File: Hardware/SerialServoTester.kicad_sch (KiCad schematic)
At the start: 12 parts, among them J1 Conn_01x04_Pin, J2 Screw_Terminal_01x02, P1 USB_C_Plug_USB2.0, Q1 BSS84, U1 FT230XS, U2 LT1785AxN8

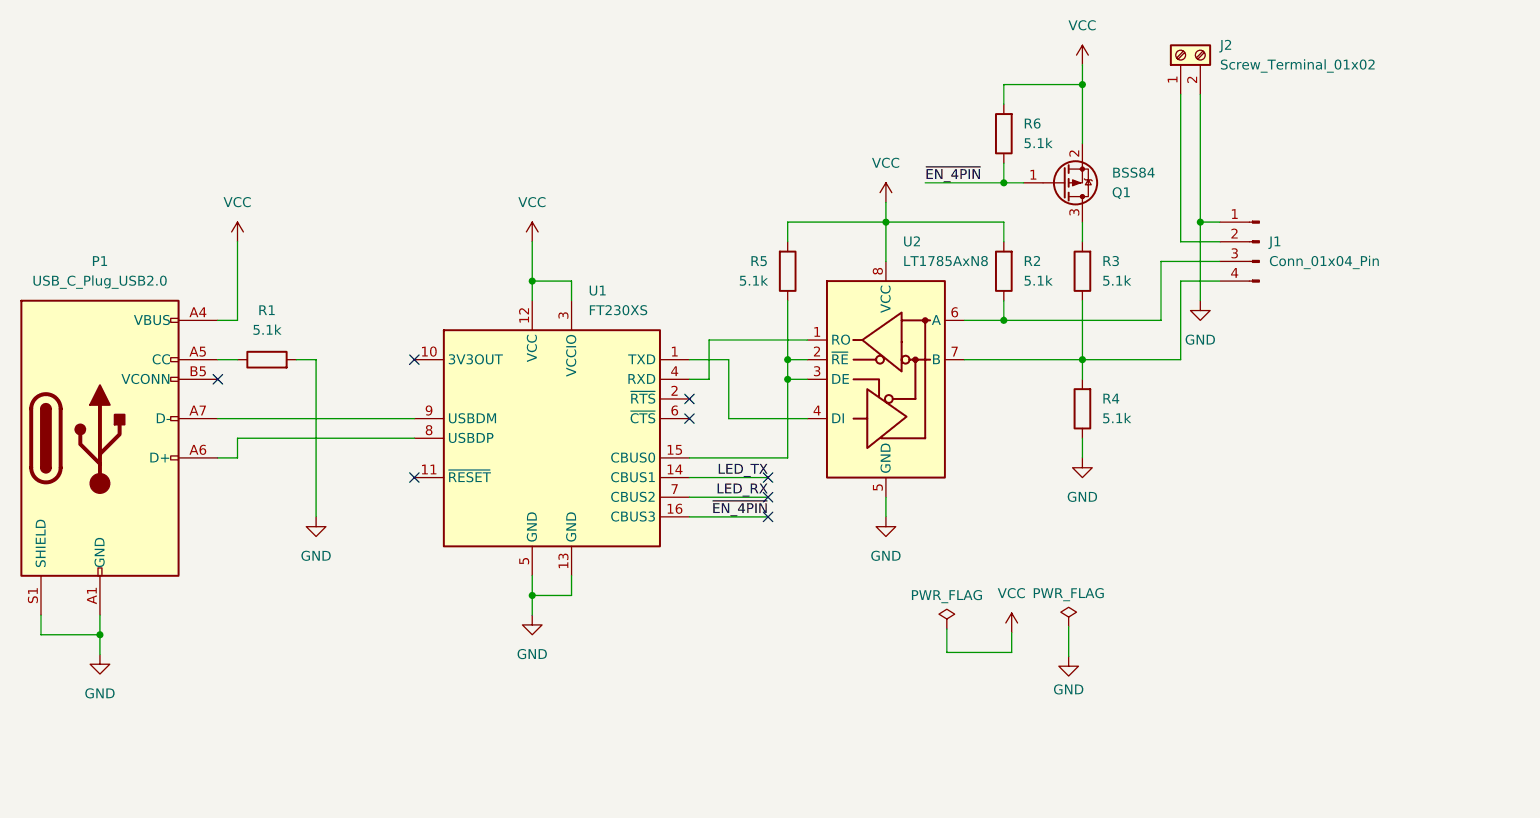
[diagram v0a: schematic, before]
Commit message: Update PCB design
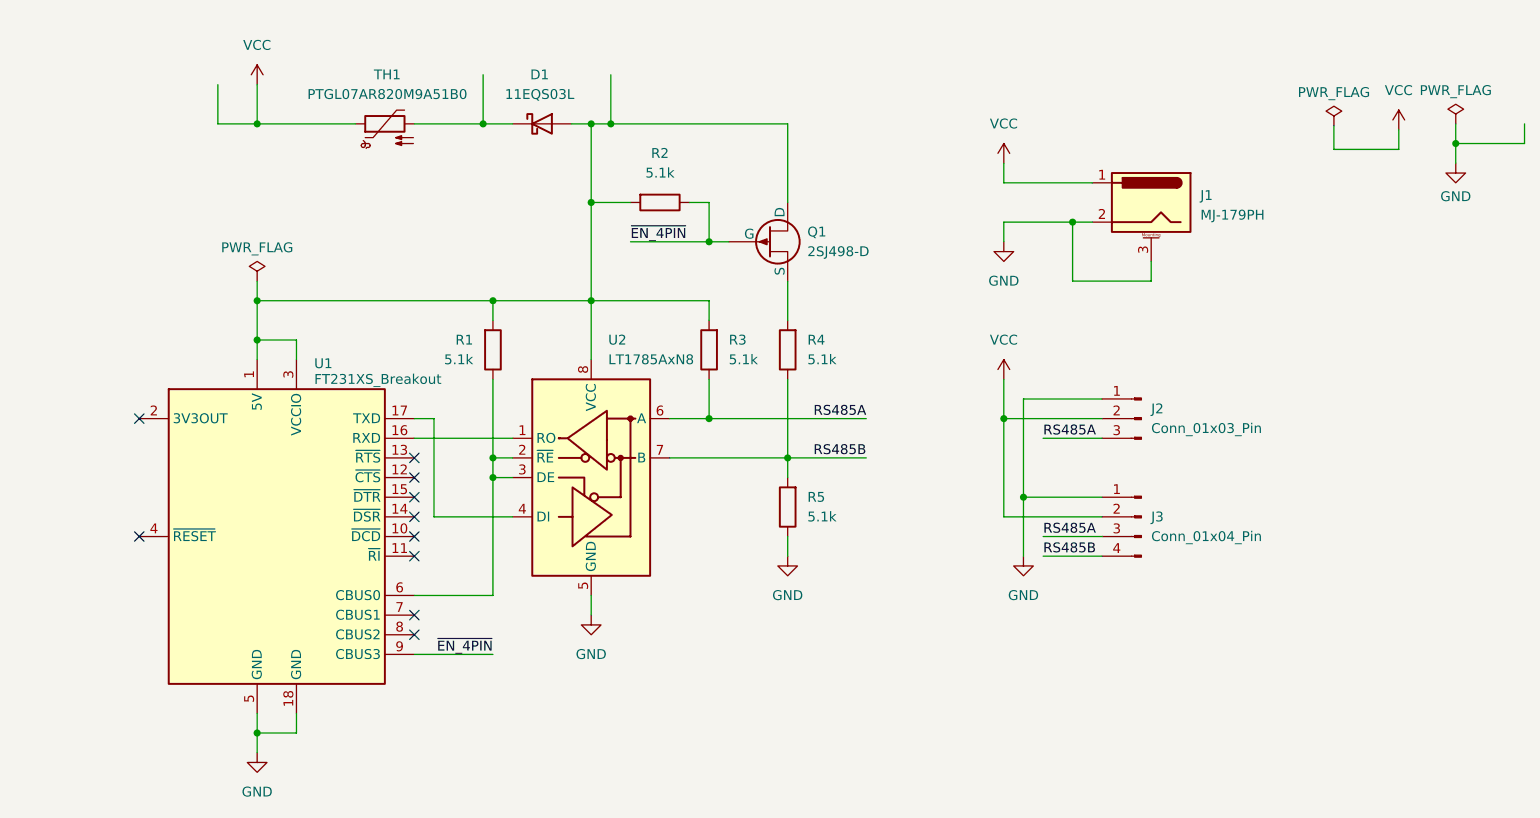
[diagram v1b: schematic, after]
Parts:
- removed J2: Screw_Terminal_01x02, TerminalBlock:TerminalBlock_bornier-2_P5.08mm, symbol Connector:Screw_Terminal_01x02
- removed P1: USB_C_Plug_USB2.0, Connector_USB:USB_C_Plug_JAE_DX07P024AJ1, symbol Connector:USB_C_Plug_USB2.0
- removed Q1: BSS84, Package_TO_SOT_SMD:SOT-23, symbol Transistor_FET:BSS84
- removed R1, R6: 5.1k, Resistor_SMD:R_0603_1608Metric_Pad0.98x0.95mm_HandSolder, symbol Device:R
- removed U1: FT230XS, Package_SO:SSOP-16_3.9x4.9mm_P0.635mm, symbol Interface_USB:FT230XS
- added D1: 11EQS03L, Diode_THT:D_T-1_P10.16mm_Horizontal, symbol Device:D_Schottky
- added J1: MJ-179PH, Connector_BarrelJack:BarrelJack_Horizontal, symbol Connector:Barrel_Jack_MountingPin
- added J2: Conn_01x03_Pin, Connector_PinHeader_2.54mm:PinHeader_1x03_P2.54mm_Horizontal, symbol Connector:Conn_01x03_Pin
- added Q1: 2SJ498-D, Package_TO_SOT_THT:TO-92S_Wide, symbol Simulation_SPICE:PJFET
- added R2: 5.1k, Resistor_THT:R_Axial_DIN0207_L6.3mm_D2.5mm_P10.16mm_Horizontal, symbol Device:R
- added TH1: PTGL07AR820M9A51B0, Capacitor_THT:C_Disc_D8.0mm_W5.0mm_P5.00mm, symbol Device:Thermistor_PTC
- added U1: FT231XS_Breakout, FootprintLibrary:DIP-18_500_ELL, symbol SymbolLibrary:FT231XS_Breakout
- J3: renamed from J1; footprint Connector_PinHeader_2.54mm:PinHeader_1x04_P2.54mm_Horizontal -> Connector_JST:JST_EH_S4B-EH_1x04_P2.50mm_Horizontal; URL (none) -> https://www.marutsu.co.jp/pc/i/46603/
- R1: renamed from R5; footprint Resistor_SMD:R_0603_1608Metric_Pad0.98x0.95mm_HandSolder -> Resistor_THT:R_Axial_DIN0207_L6.3mm_D2.5mm_P10.16mm_Horizontal
- R3: renamed from R2; footprint Resistor_SMD:R_0603_1608Metric_Pad0.98x0.95mm_HandSolder -> Resistor_THT:R_Axial_DIN0207_L6.3mm_D2.5mm_P10.16mm_Horizontal
- R4: renamed from R3; footprint Resistor_SMD:R_0603_1608Metric_Pad0.98x0.95mm_HandSolder -> Resistor_THT:R_Axial_DIN0207_L6.3mm_D2.5mm_P10.16mm_Horizontal
- R5: renamed from R4; footprint Resistor_SMD:R_0603_1608Metric_Pad0.98x0.95mm_HandSolder -> Resistor_THT:R_Axial_DIN0207_L6.3mm_D2.5mm_P10.16mm_Horizontal
- U2: footprint Package_DIP:DIP-8_W7.62mm -> Package_DIP:DIP-8_W7.62mm_Socket_LongPads; URL (none) -> https://akizukidenshi.com/catalog/g/g115806/
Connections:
- net GND: now also J1.2, J1.3 (MountPin), J2.1 (Pin_1), U1.18 (GND), U1.5 (GND)
- net VCC: now also J3.2 (Pin_2), J1.1, J2.2 (Pin_2), TH1.1; no longer R1.2, R3.2, U2.8 (VCC)
- net ~{EN_4PIN}: now also Q1.2 (G), R2.1, U1.9 (CBUS3)
- net RS485A: now reaches J3.3 (Pin_3), R3.1, U2.6 (A)
- net RS485A: now also J2.3 (Pin_3)
- net RS485B: now reaches J3.4 (Pin_4), R4.1, R5.2, U2.7 (B)
- net at R4.2: now also Q1.3 (S)
- net at R1.1, U2.2 (~{RE}), U2.3 (DE): now also U1.6 (CBUS0)
- net at U2.1 (RO): now also U1.16 (RXD)
- net at U2.4 (DI): now also U1.17 (TXD)
- new net: D1.1 (K), TH1.2
- new net: D1.2 (A), Q1.1 (D), R1.2, R2.2, R3.2, U1.1 (5V), U1.3 (VCCIO), U2.8 (VCC)
- no-connect marks 8 -> 10
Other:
- moved on the sheet: J3, R1, R3, R4, R5, U2
